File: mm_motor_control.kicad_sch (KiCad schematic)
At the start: 0 parts

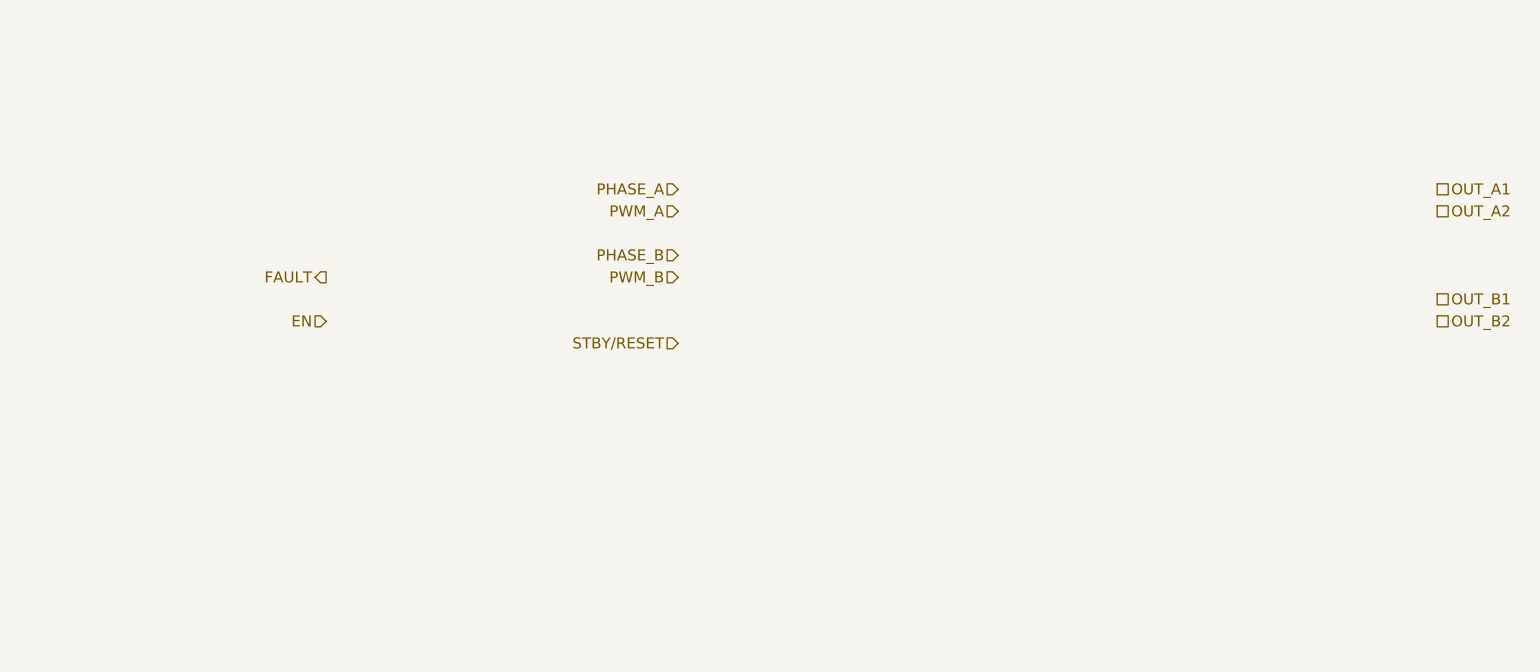
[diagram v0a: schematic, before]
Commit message: tp2
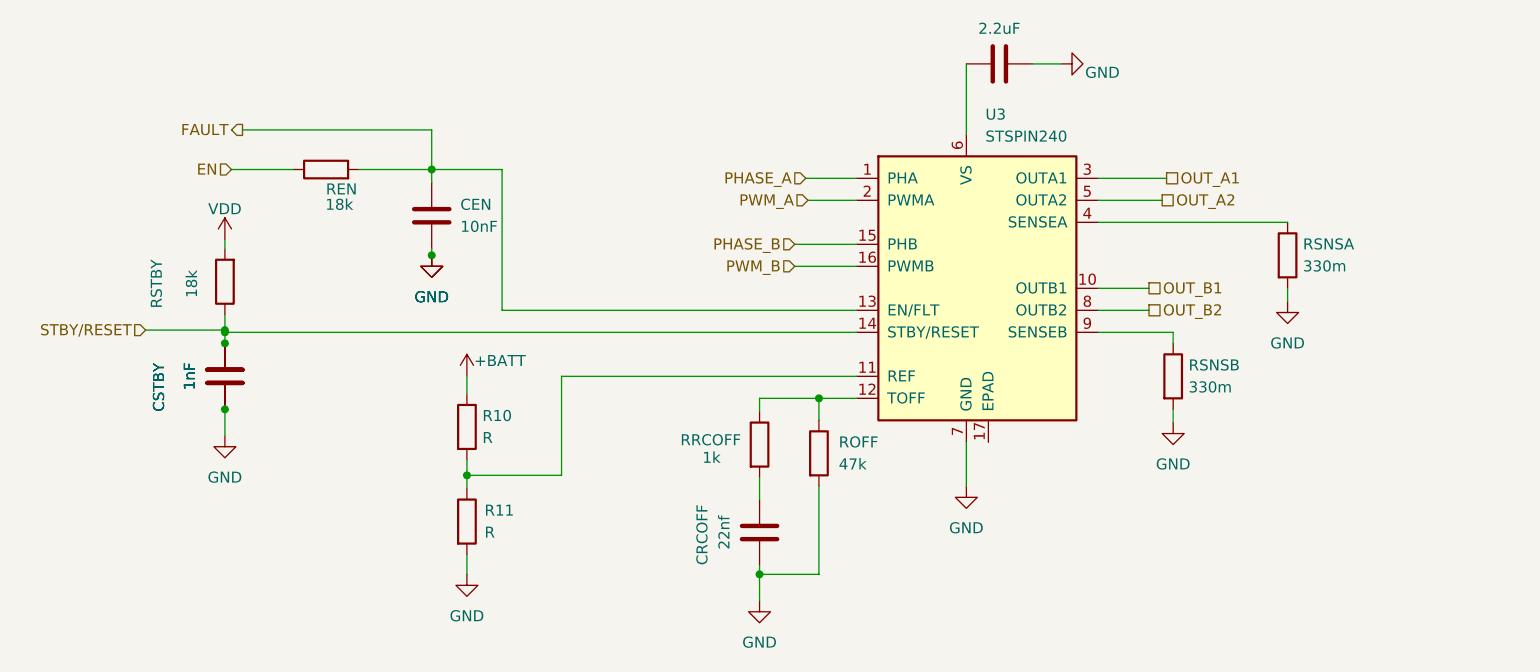
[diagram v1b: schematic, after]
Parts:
- added CEN: 10nF, symbol Device:C
- added CRCOFF: 22nf, symbol Device:C
- added CS: 2.2uF, symbol Device:C
- added CSTBY (x2): 1nF, symbol Device:C
- added R10, R11: R, symbol Device:R
- added REN, RSTBY: 18k, symbol Device:R
- added ROFF: 47k, symbol Device:R
- added RRCOFF: 1k, symbol Device:R
- added RSNSA, RSNSB: 330m, symbol Device:R
- added U3: STSPIN240, Package_DFN_QFN:VQFN-16-1EP_3x3mm_P0.5mm_EP1.8x1.8mm, symbol Driver_Motor:STSPIN240
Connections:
- net EN: now also REN.1
- net FAULT: now also CEN.1, REN.2, U3.13 (EN/FLT)
- net OUT_A1: now also U3.3 (OUTA1)
- net OUT_A2: now also U3.5 (OUTA2)
- net OUT_B1: now also U3.10 (OUTB1)
- net OUT_B2: now also U3.8 (OUTB2)
- net PHASE_A: now also U3.1 (PHA)
- net PHASE_B: now also U3.15 (PHB)
- net PWM_A: now also U3.2 (PWMA)
- net PWM_B: now also U3.16 (PWMB)
- net STBY/RESET: now also CSTBY.1, CSTBY.1, RSTBY.1, U3.14 (STBY/RESET)
- new net: ROFF.1, RRCOFF.1, U3.12 (TOFF)
- new net: CRCOFF.1, RRCOFF.2
- new net: CS.2, U3.6 (VS)
- new net: RSNSB.1, U3.9 (SENSEB)
- new net: R10.2, R11.1, U3.11 (REF)
- new net: RSNSA.1, U3.4 (SENSEA)
- new net +BATT: R10.1
- new net GND: CEN.2, CRCOFF.2, CS.1, CSTBY.2, CSTBY.2, R11.2, ROFF.2, RSNSA.2, RSNSB.2, U3.7 (GND)
- new net VDD: RSTBY.2
